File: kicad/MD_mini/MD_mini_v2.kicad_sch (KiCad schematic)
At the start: 82 parts, among them J1 Conn_01x02_Pin, J3 Conn_01x02_Pin, J4 Conn_01x02_Pin, J5 Conn_02x06_Counter_Clockwise, U1 IRS2003, U10 STM32C011F4Px, U2 SCM3723ASA, U3 IRS2003, U4 ACS711xEXLT-15AB, U6 ACS711xEXLT-15AB, U7 IRS2003, U8 IRS2003, U9 SCM3723ASA

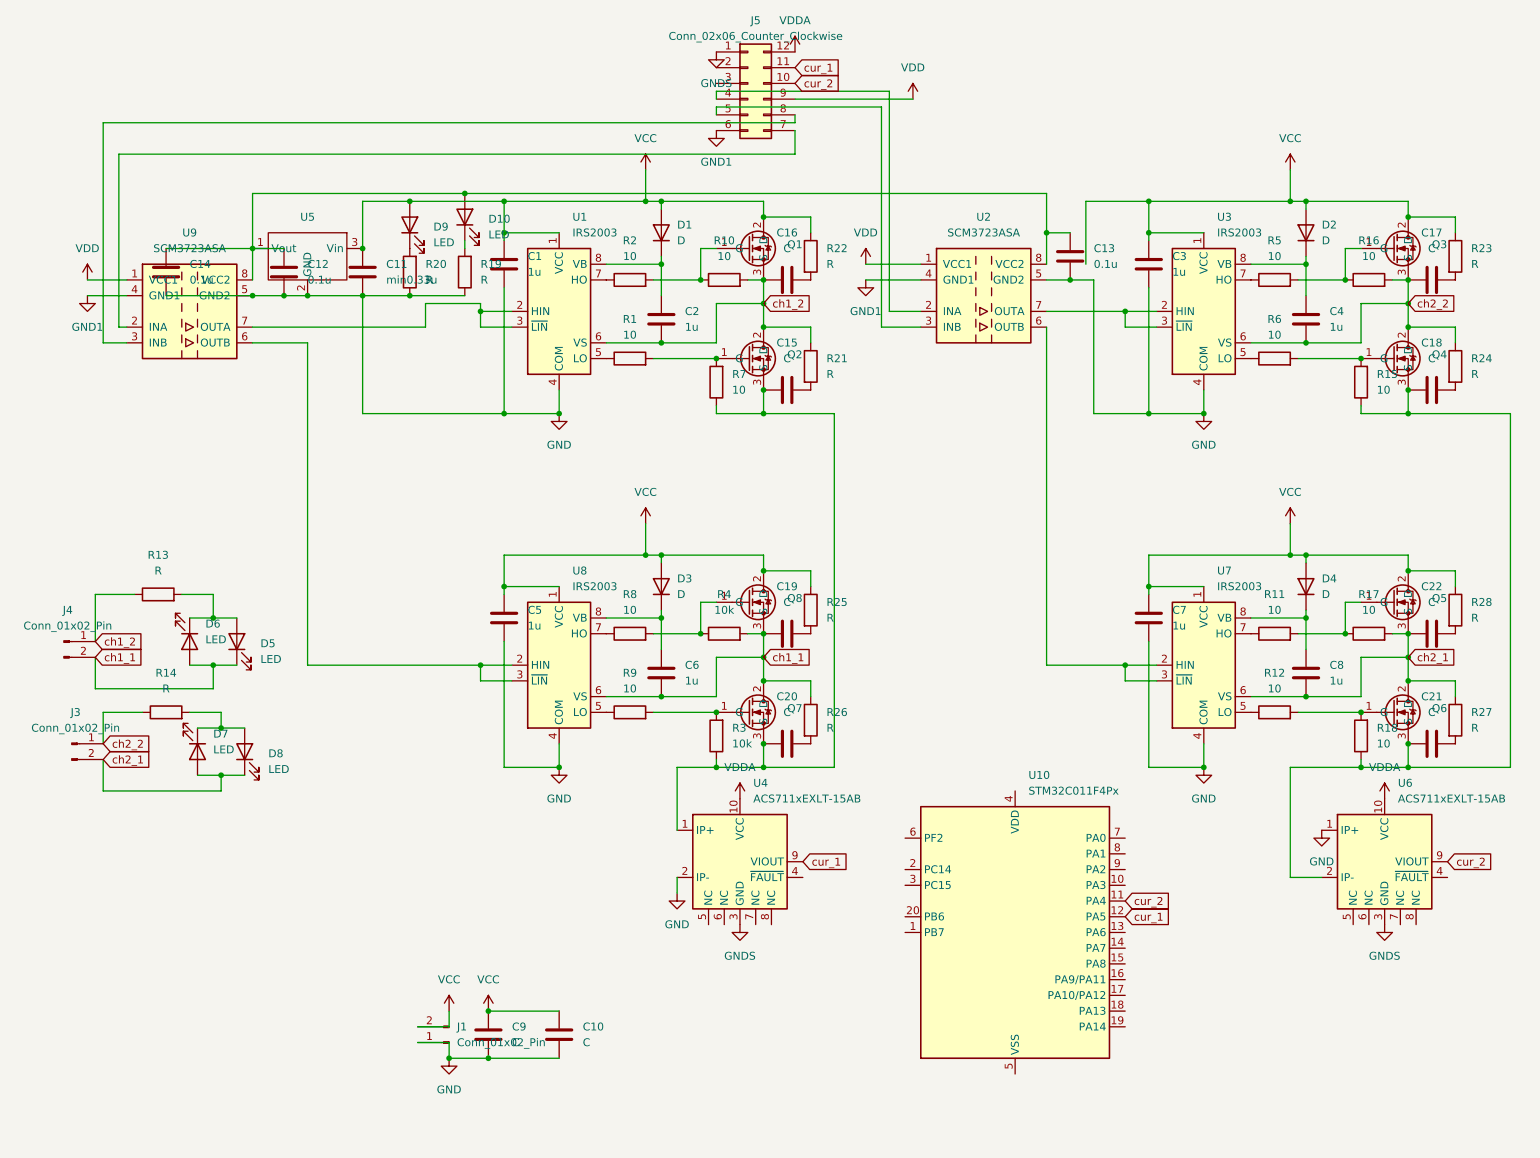
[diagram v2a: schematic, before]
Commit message: a
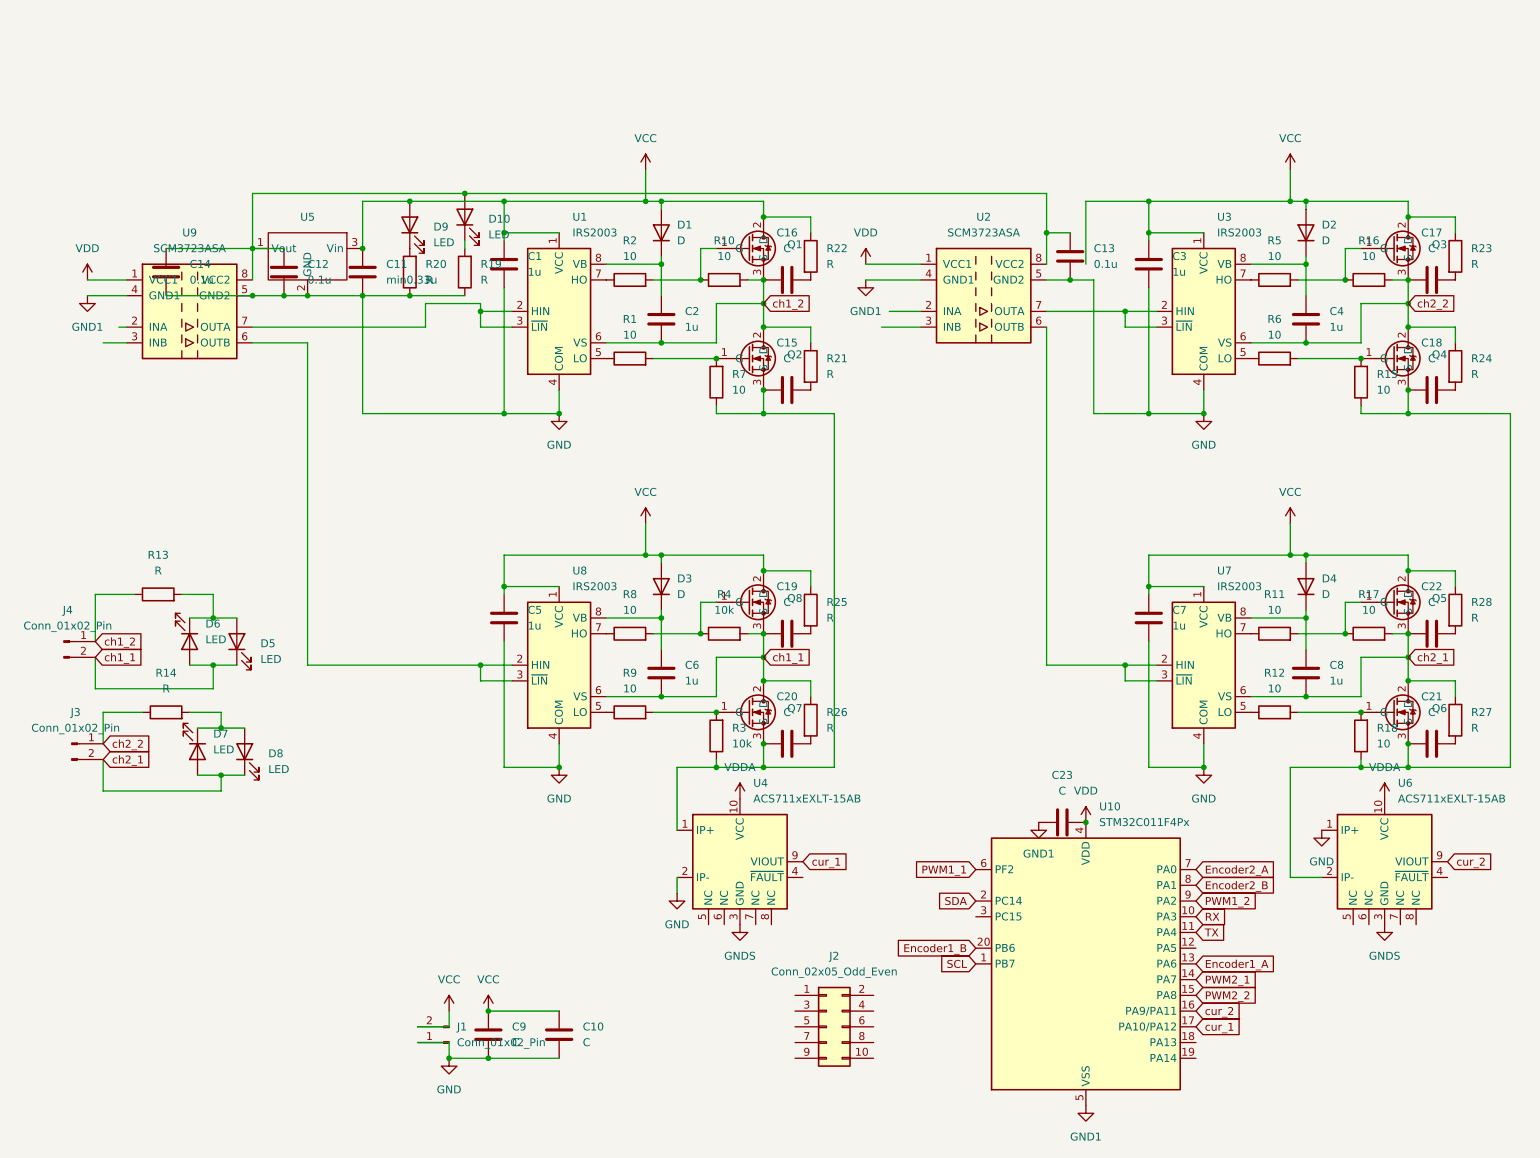
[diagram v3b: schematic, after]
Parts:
- removed J5: Conn_02x06_Counter_Clockwise, symbol Connector_Generic:Conn_02x06_Counter_Clockwise
- added C23: C, Capacitor_SMD:C_0603_1608Metric, symbol Device:C
- added J2: Conn_02x05_Odd_Even, Connector_PinHeader_2.54mm:PinHeader_2x05_P2.54mm_Horizontal, symbol Connector_Generic:Conn_02x05_Odd_Even
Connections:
- net GND1: now also U10.5 (VSS), C23.2
- net VDD: now also U10.4 (VDD), C23.1
- net cur_1: now also U10.17 (PA10/PA12); no longer U10.12 (PA5)
- net cur_2: now also U10.16 (PA9/PA11); no longer U10.11 (PA4)
- net SCL: now reaches U10.1 (PB7)
- net RX: now reaches U10.10 (PA3)
- net Encoder1_A: now reaches U10.13 (PA6)
- net PWM2_1: now reaches U10.14 (PA7)
- net PWM2_2: now reaches U10.15 (PA8)
- net SDA: now reaches U10.2 (PC14)
- net Encoder1_B: now reaches U10.20 (PB6)
- net PWM1_1: now reaches U10.6 (PF2)
- net Encoder2_A: now reaches U10.7 (PA0)
- net Encoder2_B: now reaches U10.8 (PA1)
- net PWM1_2: now reaches U10.9 (PA2)
- new net TX: U10.11 (PA4)
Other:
- moved on the sheet: U10

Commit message: a
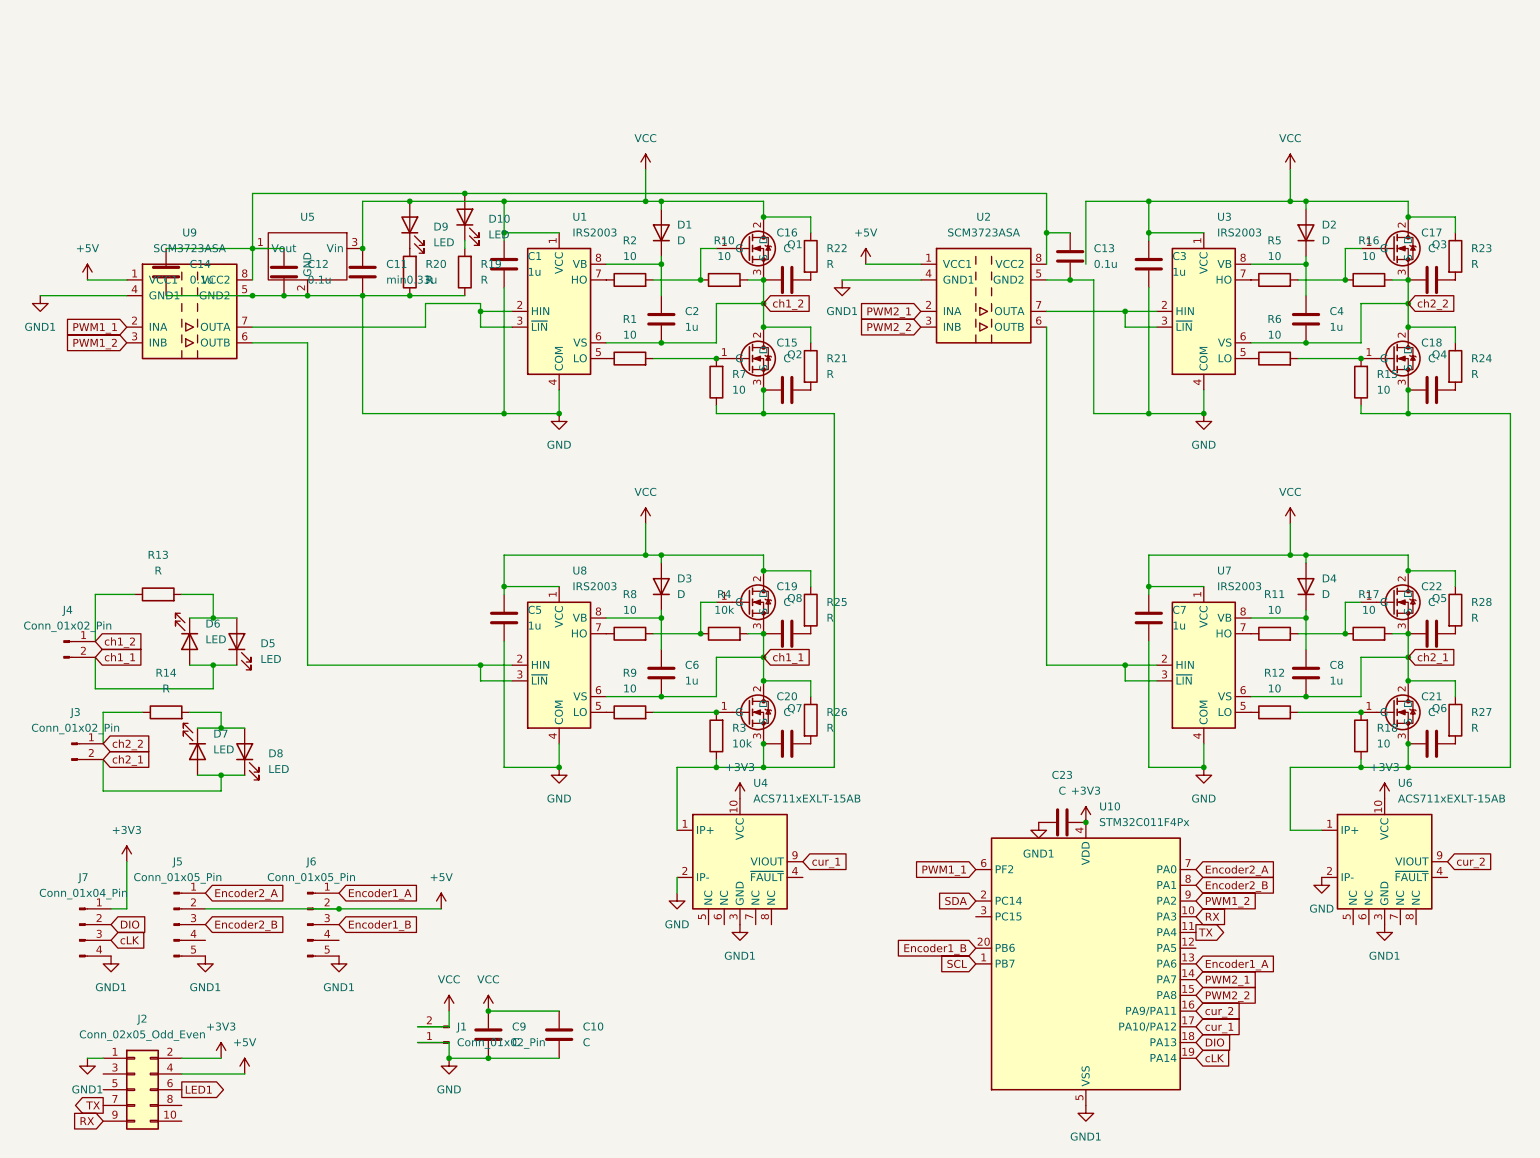
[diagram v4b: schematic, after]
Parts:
- added J5, J6: Conn_01x05_Pin, Connector_PinSocket_2.54mm:PinSocket_1x05_P2.54mm_Vertical, symbol Connector:Conn_01x05_Pin
- added J7: Conn_01x04_Pin, Connector_PinSocket_2.54mm:PinSocket_1x04_P2.54mm_Vertical, symbol Connector:Conn_01x04_Pin
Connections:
- net GNDS is gone; now on net GND1: U4.3 (GND), U6.3 (GND)
- net VDDA is gone; now on net +3V3: U4.10 (VCC), U6.10 (VCC)
- net Encoder1_A: now also J6.1 (Pin_1)
- net Encoder1_B: now also J6.3 (Pin_3)
- net Encoder2_A: now also J5.1 (Pin_1)
- net Encoder2_B: now also J5.3 (Pin_3)
- net GND: now also U6.2 (IP-); no longer U6.1 (IP+)
- net GND1: now also J2.1 (Pin_1), J5.5 (Pin_5), J6.5 (Pin_5), J7.4 (Pin_4)
- net PWM1_1: now also U9.2 (INA)
- net PWM1_2: now also U9.3 (INB)
- net PWM2_1: now also U2.2 (INA)
- net PWM2_2: now also U2.3 (INB)
- net RX: now also J2.9 (Pin_9)
- net TX: now also J2.7 (Pin_7)
- net at C18.1, C21.1, Q4.3 (S)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: now also U6.1 (IP+); no longer U6.2 (IP-)
- net +3V3: now reaches J2.2 (Pin_2)
- net +3V3: now also C23.1, U10.4 (VDD), J7.1 (Pin_1)
- net +5V: now reaches J2.4 (Pin_4)
- net +5V: now also U2.1 (VCC1), U9.1 (VCC1), J5.2 (Pin_2), J6.2 (Pin_2)
- net LED1: now reaches J2.6 (Pin_6)
- net DIO: now reaches U10.18 (PA13)
- net DIO: now also J7.2 (Pin_2)
- net cLK: now reaches U10.19 (PA14)
- net cLK: now also J7.3 (Pin_3)
- removed net VDD: C23.1, U10.4 (VDD), U2.1 (VCC1), U9.1 (VCC1)
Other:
- moved on the sheet: J2

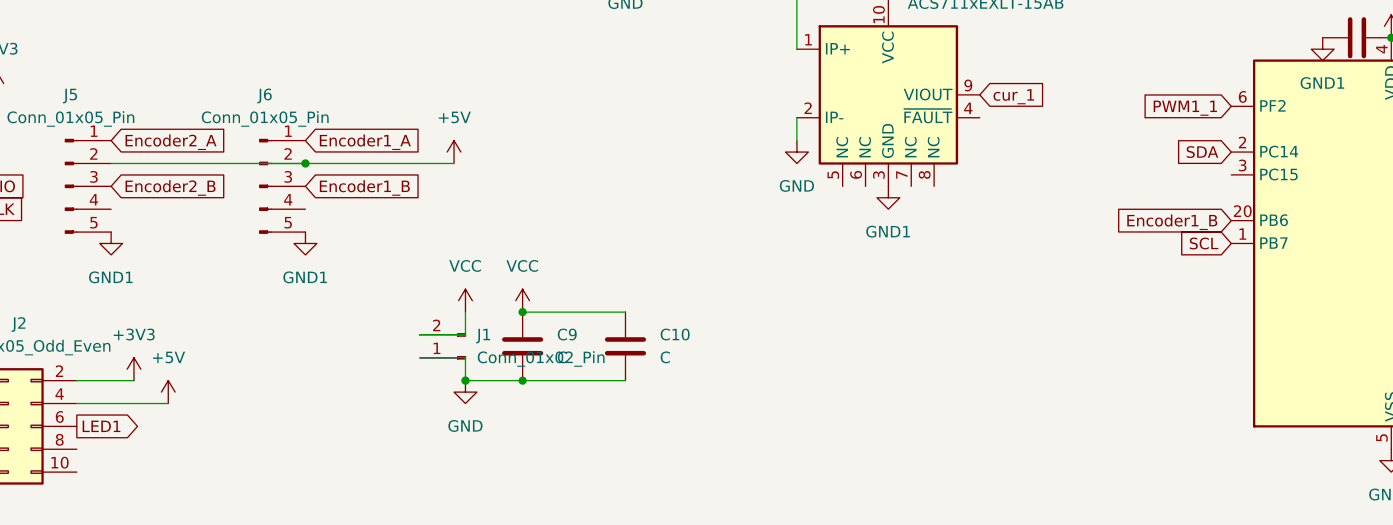
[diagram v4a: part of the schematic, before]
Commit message: a
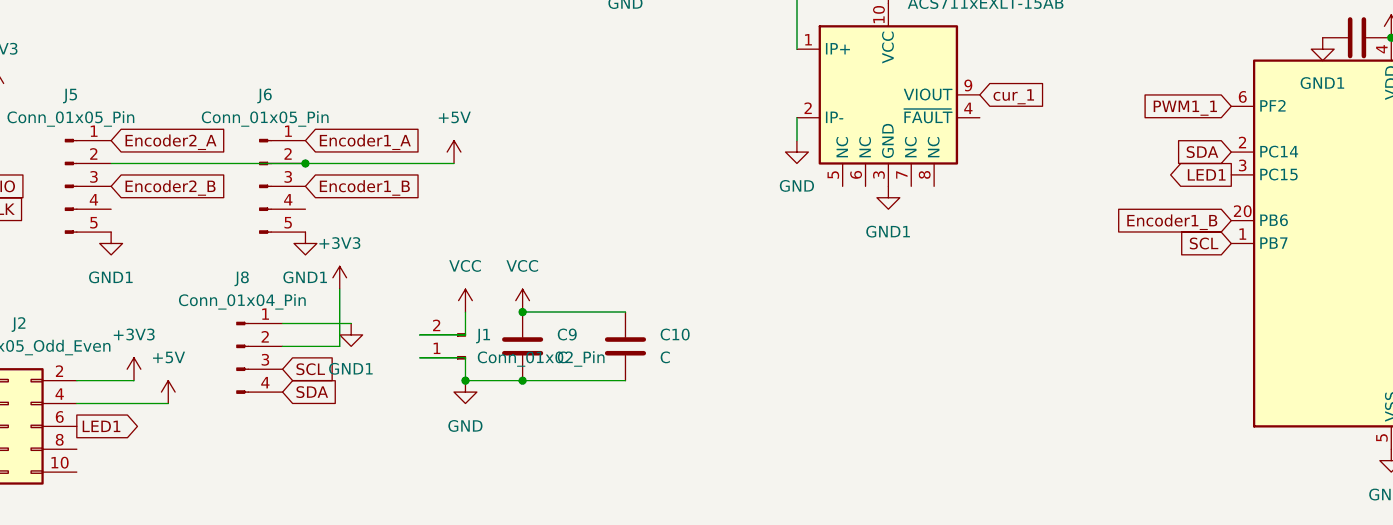
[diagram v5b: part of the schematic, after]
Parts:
- added J8: Conn_01x04_Pin, Connector_PinSocket_2.54mm:PinSocket_1x04_P2.54mm_Vertical, symbol Connector:Conn_01x04_Pin
- J5, J6: footprint Connector_PinSocket_2.54mm:PinSocket_1x05_P2.54mm_Vertical -> Connector_PinHeader_2.54mm:PinHeader_1x05_P2.54mm_Horizontal
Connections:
- net +3V3: now also J8.2 (Pin_2)
- net GND1: now also J8.1 (Pin_1)
- net LED1: now also U10.3 (PC15)
- net SCL: now also J8.3 (Pin_3)
- net SDA: now also J8.4 (Pin_4)
